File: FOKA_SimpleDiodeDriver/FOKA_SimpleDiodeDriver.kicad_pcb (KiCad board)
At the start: 2 copper layers, 30 x 30 mm, 32 parts, among them J1 IN, J2 Conn_01x02, Q2 NMOS, U1 AZ431L, U2 ADA4891-1

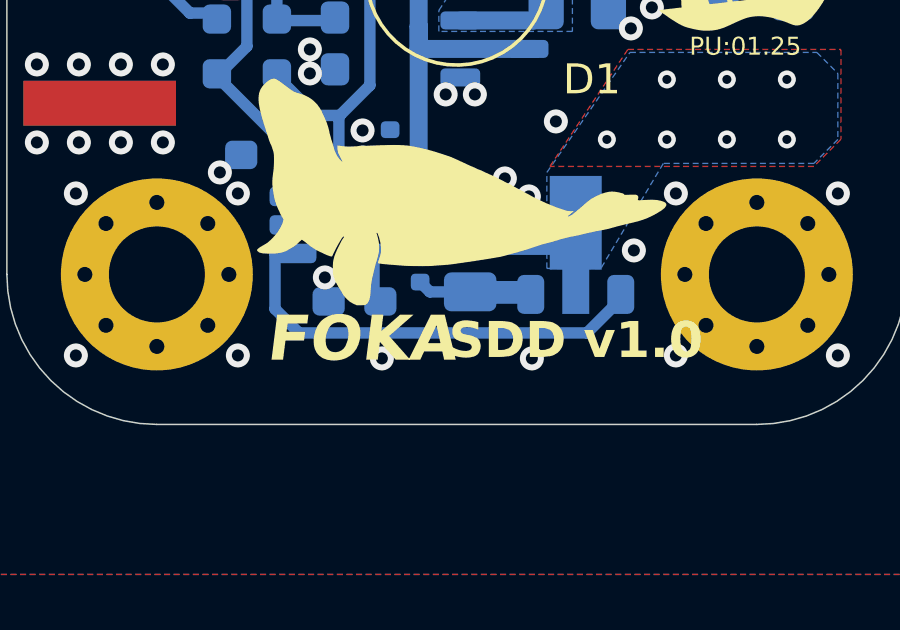
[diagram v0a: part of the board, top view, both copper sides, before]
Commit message: RezystorDoBramki
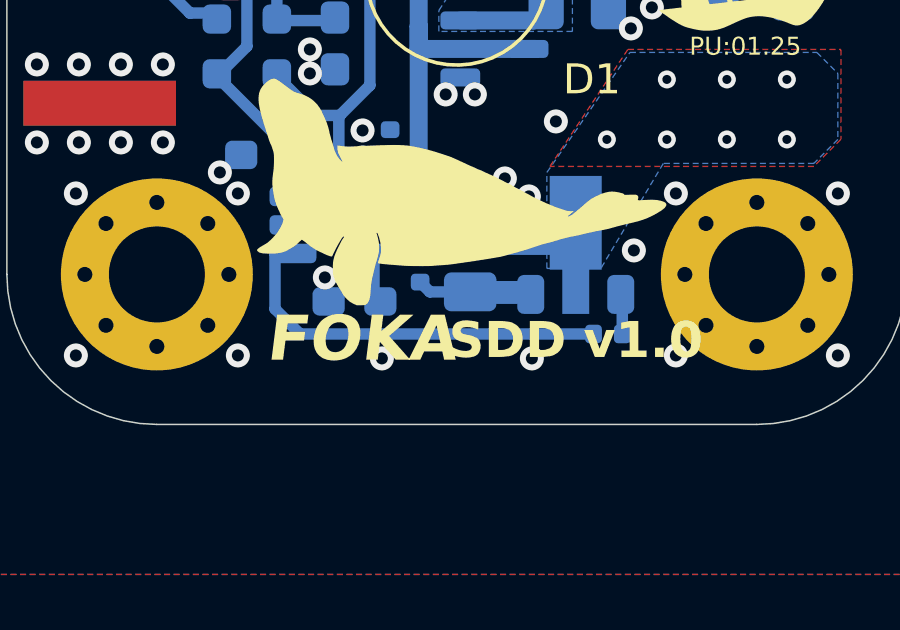
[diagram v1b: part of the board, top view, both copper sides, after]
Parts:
- added R10: optional, Capacitor_SMD:C_0402_1005Metric, B.Cu at (115.0, 72.0)
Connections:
- U2 pad 1: Net-(Q2-G) -> Net-(R10-Pad1)
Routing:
- net Net-(Q2-G): track 15.0 -> 1.53 mm
- net Net-(R10-Pad1): track 0.00 -> 13.4 mm
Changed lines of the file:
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@@
 	(net 12 "Net-(U1-REF)")
 	(net 13 "Net-(Q2-S)")
+	(net 14 "Net-(R10-Pad1)")
 	(footprint "Package_TO_SOT_THT:TO-18-2_Window"
 		(layer "F.Cu")
@@
 			(layers "B.Cu" "B.Mask" "B.Paste")
 			(roundrect_rratio 0.25)
-			(net 6 "Net-(Q2-G)")
+			(net 14 "Net-(R10-Pad1)")
 			(pintype "output")
 		)
@@
 		)
 	)
+	(footprint "Capacitor_SMD:C_0402_1005Metric"
+		(layer "B.Cu")
+		(at 115.035 71.985)
+		(descr "Capacitor SMD 0402 (1005 Metric), square (rectangular) end terminal, IPC-7351 nominal, (Body size source: IPC-SM-782 page 76, https://www.pcb-3d.com/wordpress/wp-content/uploads/ipc-sm-782a_amendment_1_and_2.pdf), generated with kicad-footprint-generator")
+		(tags "capacitor")
+		(property "Reference" "R10"
+			(at -2.335 0.015 0)
+			(layer "B.SilkS")
+			(effects
+				(font
+					(size 1 1)
+					(thickness 0.15)
+				)
+				(justify mirror)
+			)
+		)
+		(property "Value" "optional"
+			(at 0 -1.16 0)
+			(layer "B.Fab")
+			(effects
+				(font
+					(size 1 1)
+					(thickness 0.15)
+				)
+				(justify mirror)
+			)
+		)
+		(property "Datasheet" ""
+			(at 0 0 0)
+			(layer "B.Fab")
+			(hide yes)
+			(effects
+				(font
+					(size 1.27 1.27)
+					(thickness 0.15)
+				)
+				(justify mirror)
+			)
+		)
+		(property "Description" "Resistor"
+			(at 0 0 0)
+			(layer "B.Fab")
+			(hide yes)
+			(effects
+				(font
+					(size 1.27 1.27)
+					(thickness 0.15)
+				)
+				(justify mirror)
+			)
+		)
+		(property ki_fp_filters "R_*")
+		(sheetname "/")
+		(sheetfile "FOKA_SimpleDiodeDriver.kicad_sch")
+		(attr smd)
+		(fp_line
+			(start -0.107836 -0.36)
+			(end 0.107836 -0.36)
+			(stroke
+				(width 0.12)
+				(type solid)
+			)
+			(layer "B.SilkS")
+		)
+		(fp_line
+			(start -0.107836 0.36)
+			(end 0.107836 0.36)
+			(stroke
+				(width 0.12)
+				(type solid)
+			)
+			(layer "B.SilkS")
+		)
+		(fp_line
+			(start -0.91 -0.46)
+			(end -0.91 0.46)
+			(stroke
+				(width 0.05)
+				(type solid)
+			)
+			(layer "B.CrtYd")
+		)
+		(fp_line
+			(start -0.91 0.46)
+			(end 0.91 0.46)
+			(stroke
+				(width 0.05)
+				(type solid)
+			)
+			(layer "B.CrtYd")
+		)
+		(fp_line
+			(start 0.91 -0.46)
+			(end -0.91 -0.46)
+			(stroke
+				(width 0.05)
+				(type solid)
+			)
+			(layer "B.CrtYd")
+		)
+		(fp_line
+			(start 0.91 0.46)
+			(end 0.91 -0.46)
+			(stroke
+				(width 0.05)
+				(type solid)
+			)
+			(layer "B.CrtYd")
+		)
+		(fp_line
+			(start -0.5 -0.25)
+			(end -0.5 0.25)
+			(stroke
+				(width 0.1)
+				(type solid)
+			)
+			(layer "B.Fab")
+		)
+		(fp_line
+			(start -0.5 0.25)
+			(end 0.5 0.25)
+			(stroke
+				(width 0.1)
+				(type solid)
+			)
+			(layer "B.Fab")
+		)
+		(fp_line
+			(start 0.5 -0.25)
+			(end -0.5 -0.25)
+			(stroke
+				(width 0.1)
+				(type solid)
+			)
+			(layer "B.Fab")
+		)
+		(fp_line
+			(start 0.5 0.25)
+			(end 0.5 -0.25)
+			(stroke
+				(width 0.1)
+				(type solid)
+			)
+			(layer "B.Fab")
+		)
+		(fp_text user "${REFERENCE}"
+			(at 0 0 0)
+			(layer "B.Fab")
+			(effects
+				(font
+					(size 0.25 0.25)
+					(thickness 0.04)
+				)
+				(justify mirror)
+			)
+		)
+		(pad "1" smd roundrect
+			(at -0.48 0)
+			(size 0.56 0.62)
+			(layers "B.Cu" "B.Mask" "B.Paste")
+			(roundrect_rratio 0.25)
+			(net 14 "Net-(R10-Pad1)")
+			(pintype "passive")
+		)
+		(pad "2" smd roundrect
+			(at 0.48 0)
+			(size 0.56 0.62)
+			(layers "B.Cu" "B.Mask" "B.Paste")
+			(roundrect_rratio 0.25)
+			(net 6 "Net-(Q2-G)")
+			(pintype "passive")
+		)
+		(embedded_fonts no)
+		(model "${KICAD9_3DMODEL_DIR}/Capacitor_SMD.3dshapes/C_0402_1005Metric.step"
+			(offset
+				(xyz 0 0 0)
+			)
+			(scale
+				(xyz 1 1 1)
+			)
+			(rotate
+				(xyz 0 0 0)
+			)
+		)
+	)
 	(footprint "Resistor_SMD:R_0603_1608Metric_Pad0.98x0.95mm_HandSolder"
 		(layer "B.Cu")
@@
 	)
 	(segment
-		(start 103.9375 71.15)
-		(end 104.7375 71.95)
-		(width 0.381)
-		(layer "B.Cu")
-		(net 6)
-	)
-	(segment
-		(start 103.9375 69.3)
-		(end 103.9375 71.15)
-		(width 0.381)
-		(layer "B.Cu")
-		(net 6)
-	)
-	(segment
-		(start 104.7375 71.95)
-		(end 114.3375 71.95)
+		(start 115.515 70.718843)
+		(end 115.4625 70.666343)
 		(width 0.381)
 		(layer "B.Cu")
@@
 	)
 	(segment
-		(start 115.5 70.7875)
-		(end 115.5 70.6)
-		(width 0.381)
-		(layer "B.Cu")
-		(net 6)
-	)
-	(segment
-		(start 104.5375 69.3)
-		(end 103.9375 69.3)
+		(start 115.5 70.6)
+		(end 115.5 70.7875)
 		(width 0.381)
 		(layer "B.Cu")
@@
 	)
 	(segment
-		(start 114.3375 71.95)
-		(end 115.5 70.7875)
+		(start 115.515 71.985)
+		(end 115.515 70.718843)
 		(width 0.381)
 		(layer "B.Cu")
@@
 		(net 13)
 	)
+	(segment
+		(start 103.9375 71.15)
+		(end 104.7725 71.985)
+		(width 0.381)
+		(layer "B.Cu")
+		(net 14)
+	)
+	(segment
+		(start 104.5375 69.3)
+		(end 103.9375 69.3)
+		(width 0.381)
+		(layer "B.Cu")
+		(net 14)
+	)
+	(segment
+		(start 104.7725 71.985)
+		(end 114.555 71.985)
+		(width 0.381)
+		(layer "B.Cu")
+		(net 14)
+	)
+	(segment
+		(start 103.9375 69.3)
+		(end 103.9375 71.15)
+		(width 0.381)
+		(layer "B.Cu")
+		(net 14)
+	)
 	(zone
